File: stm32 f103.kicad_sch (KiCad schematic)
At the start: 67 parts, among them J1 USB_C_Receptacle_USB2.0_14P, J2 Screw_Terminal_01x02, J3 Screw_Terminal_01x12, J4 Screw_Terminal_01x14, J5 Screw_Terminal_01x04, J6 Screw_Terminal_01x08, SW1 SW_Push, SW2 SW_SPDT, U1 STM32F103C6Tx, U2 PAC1934x-xJ6CX, U4 USBLC6-2SC6, U5 LD3985M33R_SOT23, U6 MCP2551-I-P, Y1 16Mhz

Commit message: final sch
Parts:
- J5: footprint (none) -> Connector_Phoenix_MC:PhoenixContact_MCV_1,5_4-G-3.5_1x04_P3.50mm_Vertical
- J6: footprint (none) -> Connector_Phoenix_MC:PhoenixContact_MCV_1,5_8-G-3.81_1x08_P3.81mm_Vertical
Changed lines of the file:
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@@
 			)
 		)
-		(property "Footprint" ""
+		(property "Footprint" "Connector_Phoenix_MC:PhoenixContact_MCV_1,5_8-G-3.81_1x08_P3.81mm_Vertical"
 			(at 284.48 199.39 0)
 			(hide yes)
@@
 			)
 		)
-		(property "Footprint" ""
+		(property "Footprint" "Connector_Phoenix_MC:PhoenixContact_MCV_1,5_4-G-3.5_1x04_P3.50mm_Vertical"
 			(at 341.63 198.12 0)
 			(hide yes)

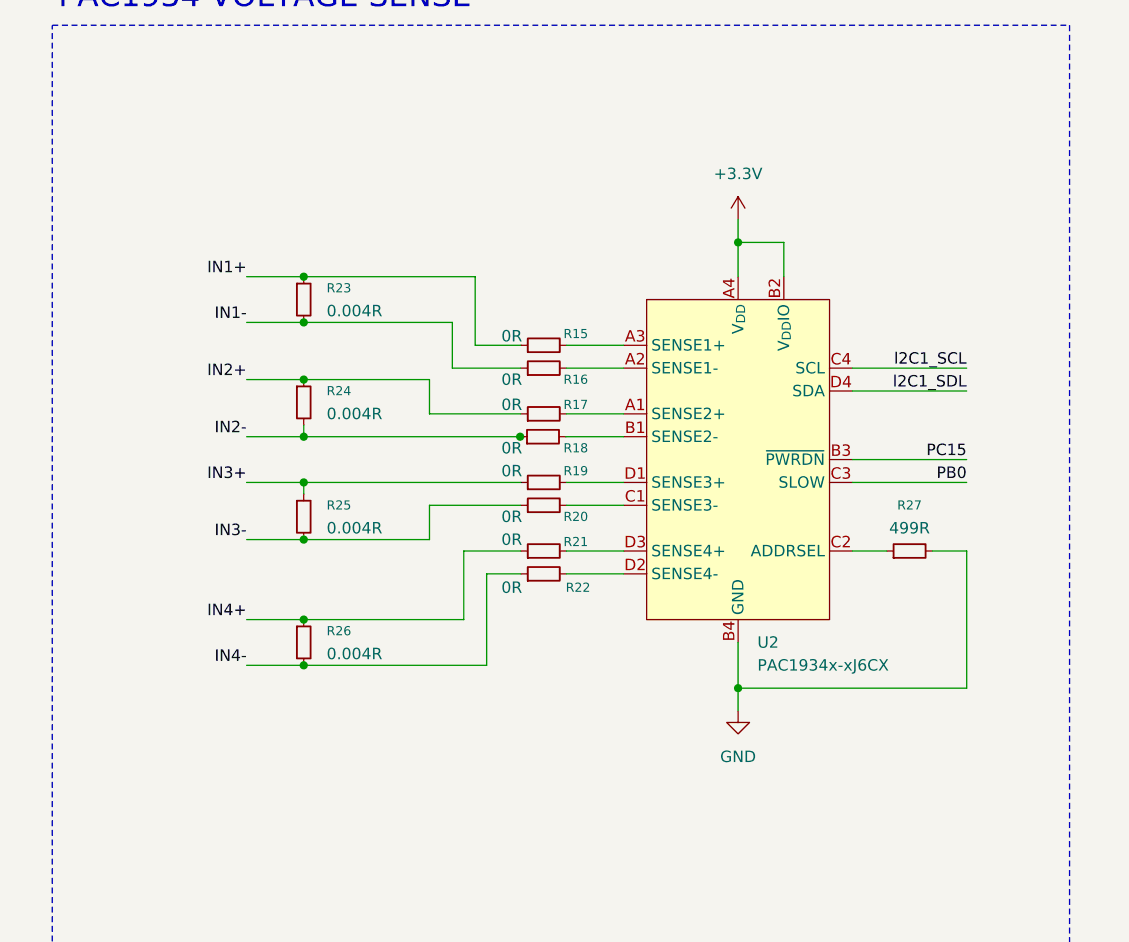
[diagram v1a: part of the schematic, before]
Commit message: for ic going for new file
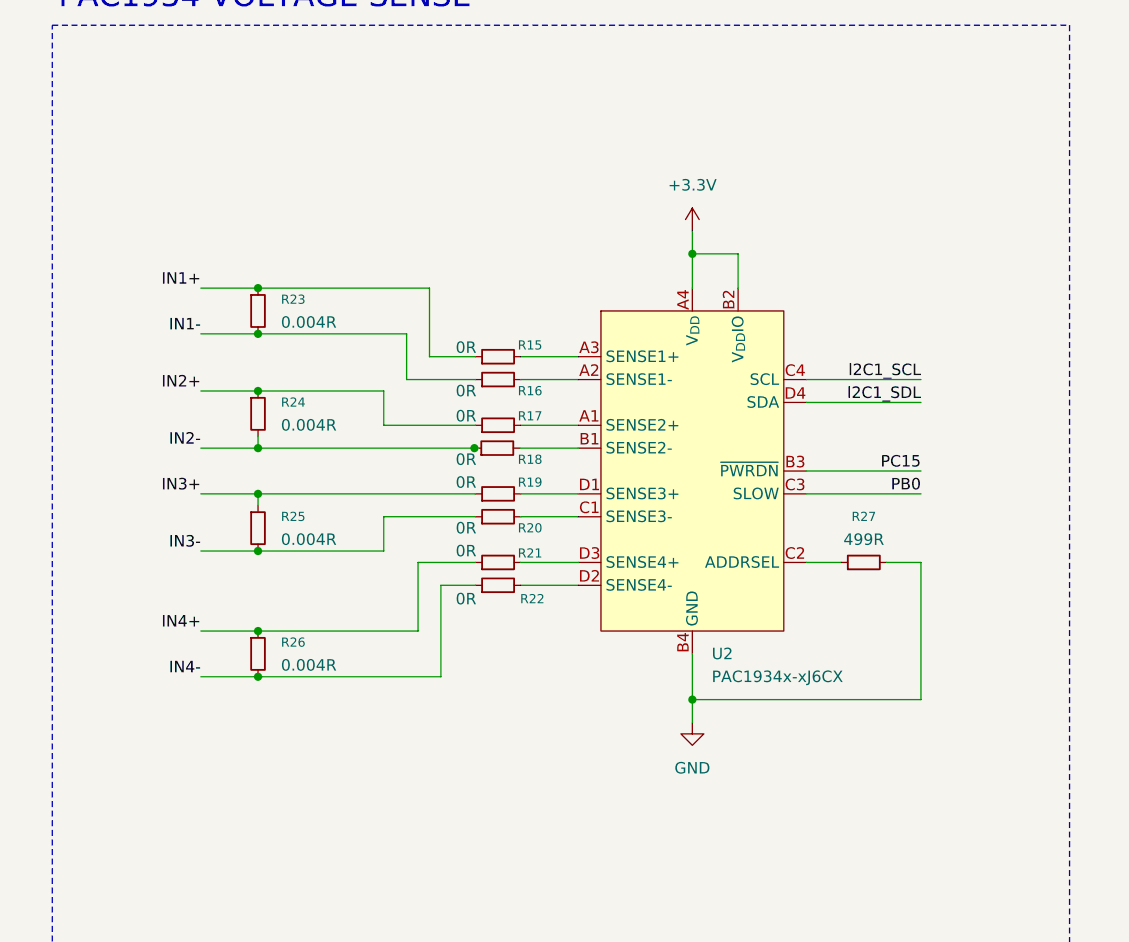
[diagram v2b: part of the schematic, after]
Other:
- moved on the sheet: R15, R16, R17, R18, R19, R20, R21, R22, R23, R24, R25, R26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
